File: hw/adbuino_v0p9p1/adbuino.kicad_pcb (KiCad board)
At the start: 2 copper layers, 25 x 50 mm, 74 parts, among them IC1 MAX3421EEHJ+, J1 Conn_01x06_Male, J2 U254-051N-4BH806, J3 USB_A, J4 Mini-DIN-4, J5 Mini-DIN-4, Q1 BSS138, Q2 BSS138, U1 AMS1117-3.3, U2 ATmega328P-AU, Y1 16MHz, Y2 12MHz

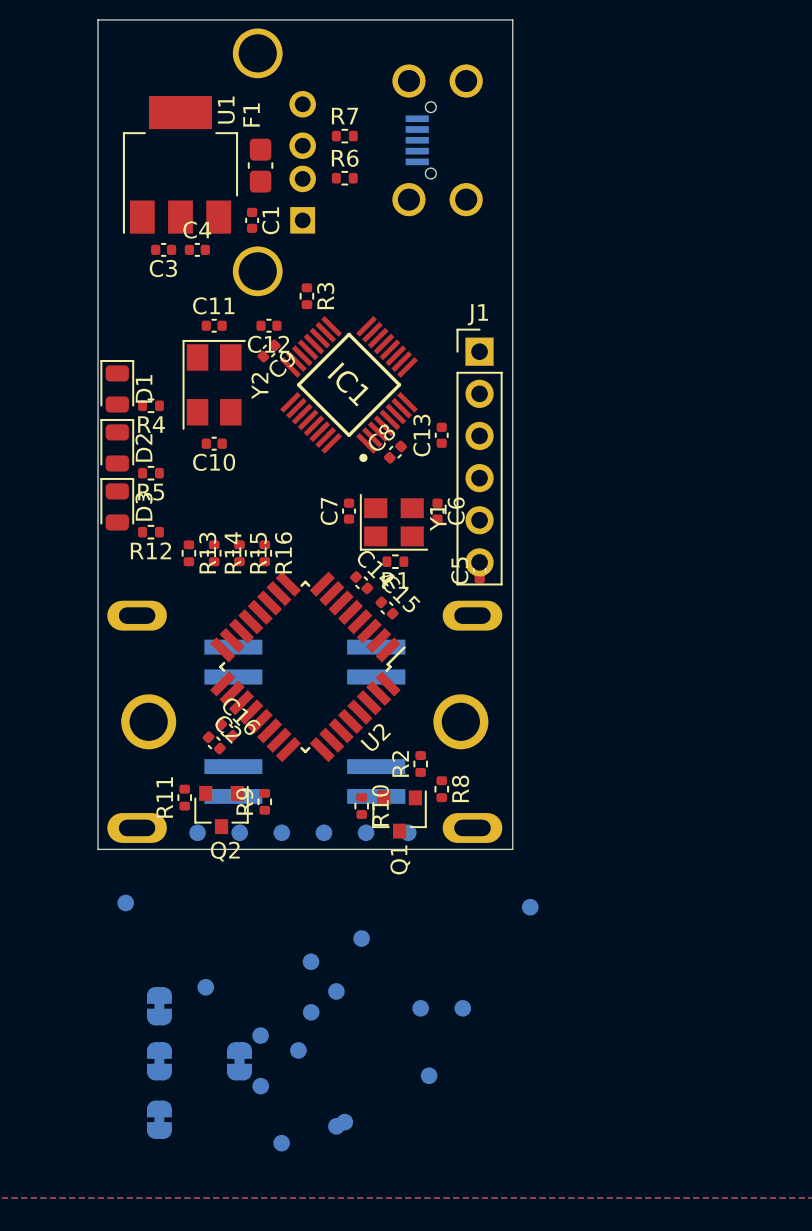
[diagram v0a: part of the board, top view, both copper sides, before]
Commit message: updates
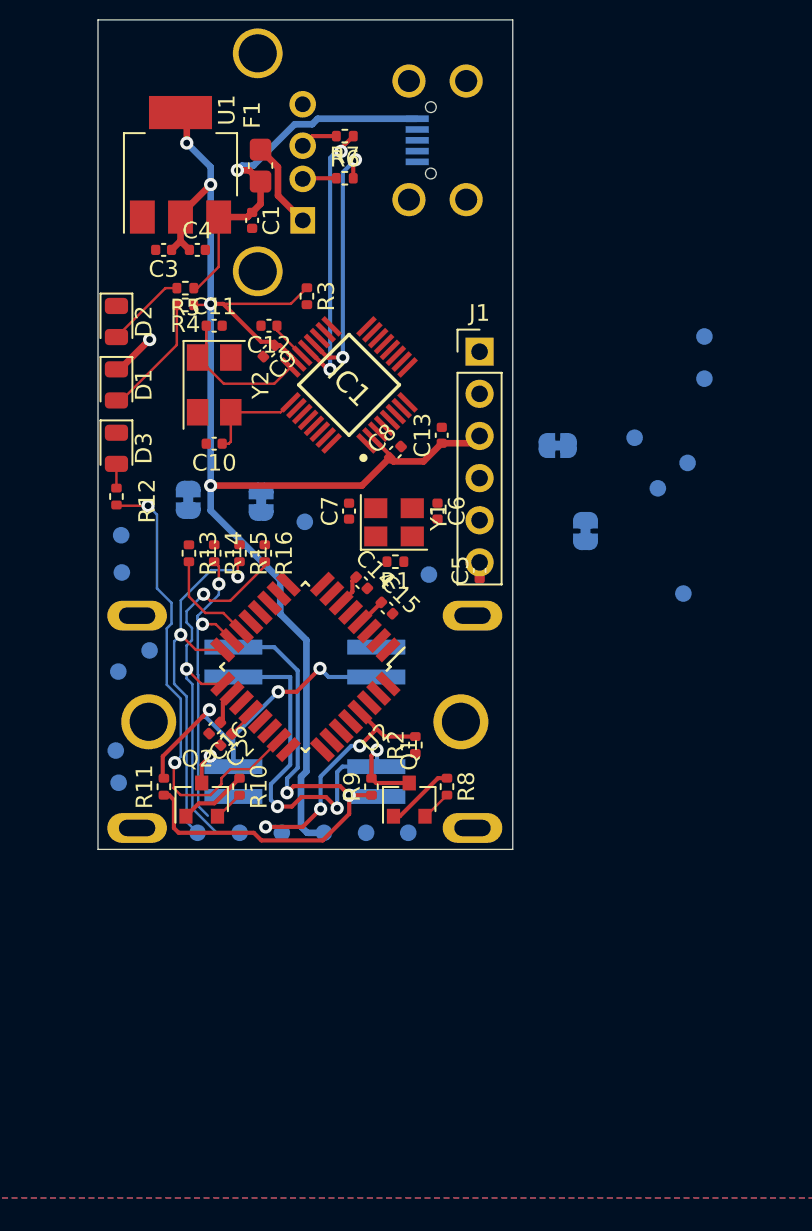
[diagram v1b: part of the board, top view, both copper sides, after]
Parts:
- removed TP10, TP9: TestPoint_Small, TestPoint:TestPoint_Pad_D1.0mm
- moved JP6 44.2 mm to (52.7, 50.7), turned to 0 degrees
- moved TP15 43.0 mm to (61.6, 44.1), turned to 0 degrees
- moved TP17 41.6 mm to (61.6, 46.6), turned to 180 degrees
- moved TP3 38.3 mm to (60.5, 51.7), turned to 0 degrees
- moved JP3 38.2 mm to (54.4, 55.8)
- moved JP4 37.8 mm to (34.8, 54.0)
- moved TP5 37.3 mm to (60.3, 59.6), turned to 0 degrees
- moved TP16 36.5 mm to (37.5, 55.3)
- moved TP13 35.4 mm to (58.7, 53.2), turned to 180 degrees
- moved TP11 34.4 mm to (57.3, 50.2), turned to 180 degrees
- moved TP4 32.8 mm to (26.4, 56.1)
- moved TP7 30.8 mm to (28.1, 63.0)
- moved JP5 30.6 mm to (30.4, 53.9), turned to 90 degrees
- moved TP8 30.1 mm to (26.2, 64.3)
- moved TP12 29.6 mm to (44.9, 58.4)
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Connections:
- IC1 pad 15: SPI_MISO -> (no net)
- TP14 pad 1: SPI_MISO -> ATMEGA_SPI_MISO
- TP22 pad 1: (no net) -> ATMEGA_SPI_SCLK
- TP25 pad 1: (no net) -> ATMEGA_SPI_MOSI
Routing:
- net +3V3: track 0.00 -> 91.7 mm, vias 0 -> 4
- net ADB_1_5v: track 0.00 -> 34.3 mm, vias 0 -> 2
- net DEBUG_LED: track 0.00 -> 28.3 mm, vias 0 -> 2
- net ADB_1_DATA: track 0.00 -> 25.9 mm, vias 0 -> 3
- net ADB_1_PWR_ON: track 0.00 -> 25.8 mm, vias 0 -> 4
- net ATMEGA_SPI_SCLK: track 0.00 -> 24.8 mm, vias 0 -> 2
- net VBUS: track 0.00 -> 23.0 mm, vias 0 -> 1
- net ATMEGA_SPI_MISO: track 0.00 -> 23.0 mm, vias 0 -> 2
- net ATMEGA_SPI_MOSI: track 0.00 -> 19.0 mm, vias 0 -> 2
- net Host_USB_D+: track 0.00 -> 16.6 mm, vias 0 -> 2
- net Host_USB_D-: track 0.00 -> 15.5 mm, vias 0 -> 2
- net /RESET: track 0.00 -> 15.4 mm, vias 0 -> 3
- net Net-(C11-Pad1): track 0.00 -> 8.79 mm
- net VCC: track 0.00 -> 8.35 mm
- net Net-(D1-Pad2): track 0.00 -> 7.49 mm
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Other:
- rule trace_min: 0.2 -> 0.15
